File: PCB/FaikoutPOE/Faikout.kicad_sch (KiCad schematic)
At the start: 83 parts, among them J1 RJ45_LED, J3 S21, J5 Reset, J7 TC2030-USB-NL-DS, M1 Ag9912-LP, P1 Square, Q1 BSS138PS, Q2 BSS138PS, U1 KSZ8851SNL, U2 ESP32-S3-MINI-1, U3 TCMT1100, U4 TPS62933, U5 TCMT1100, Y1 Crystal_GND24

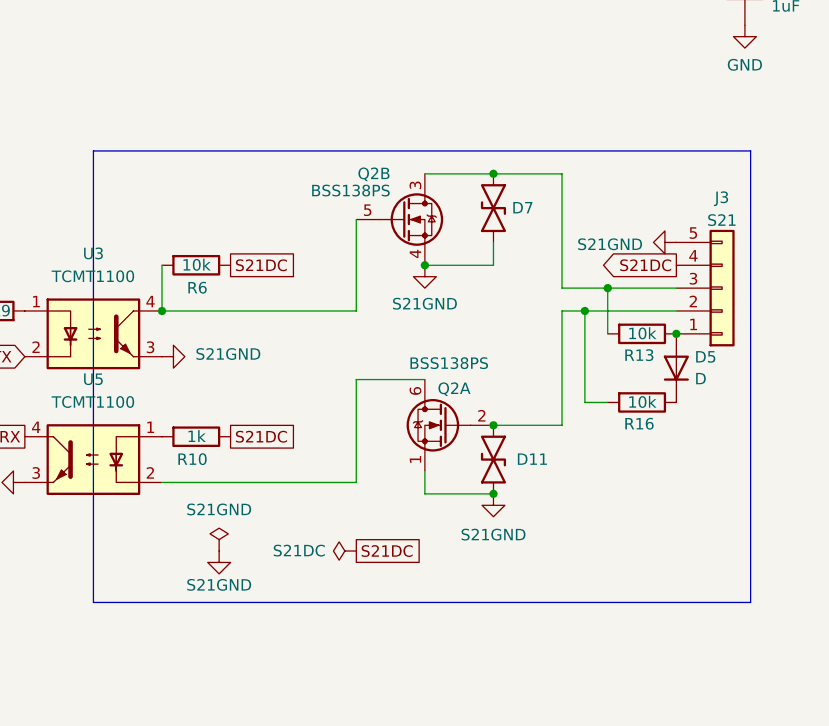
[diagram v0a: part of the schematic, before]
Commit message: Tweak
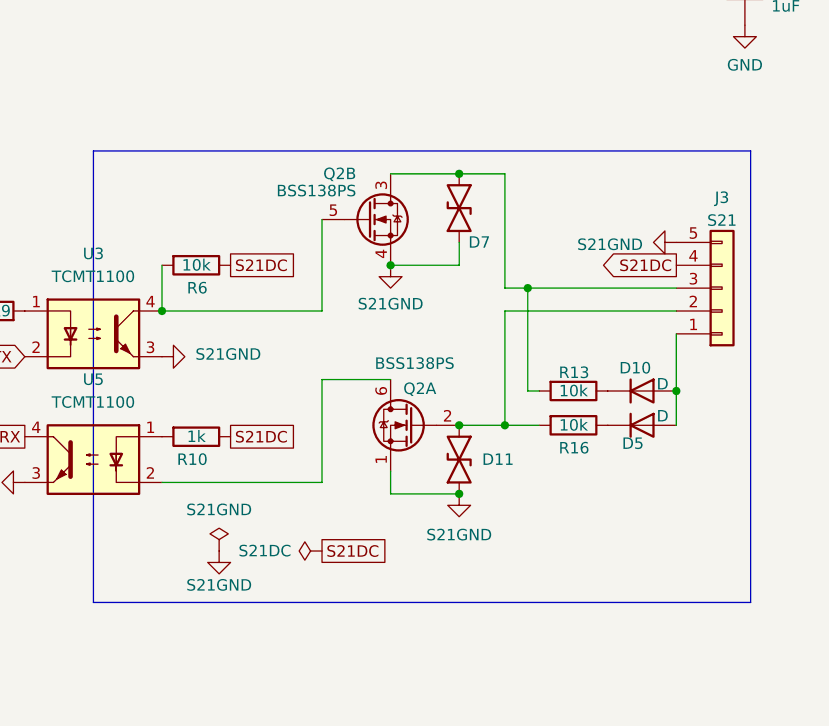
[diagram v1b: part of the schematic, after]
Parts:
- added D10: D, RevK:D_0402, symbol Device:D
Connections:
- net at D5.2 (A), J3.1 (Pin_1): now also D10.2 (A); no longer R13.1
- new net: D10.1 (K), R13.1
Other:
- moved on the sheet: D11, D5, D7, Q2A, Q2B, R13, R16
